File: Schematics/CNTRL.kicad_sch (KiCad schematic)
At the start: 14 parts, among them SW1 RotaryEncoder_Switch, SW2 RotaryEncoder_Switch, SW3 RotaryEncoder_Switch, U5 MCP23017_SP

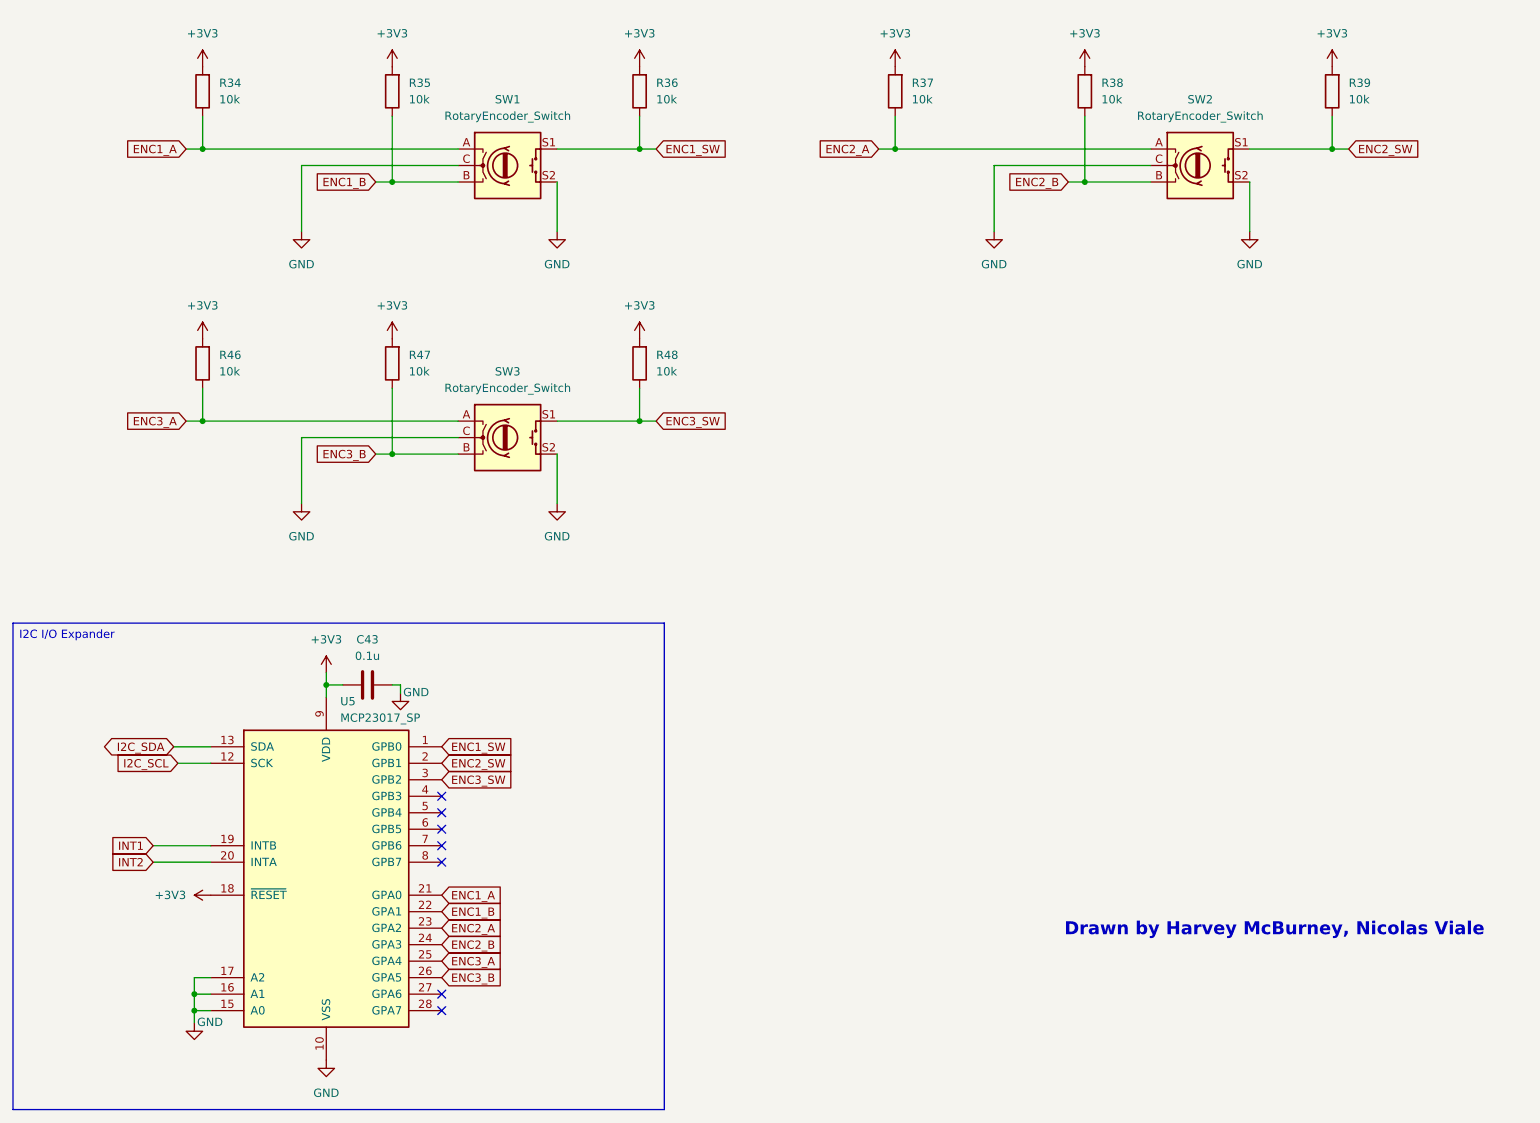
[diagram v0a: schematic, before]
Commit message: Tidied up Schematic
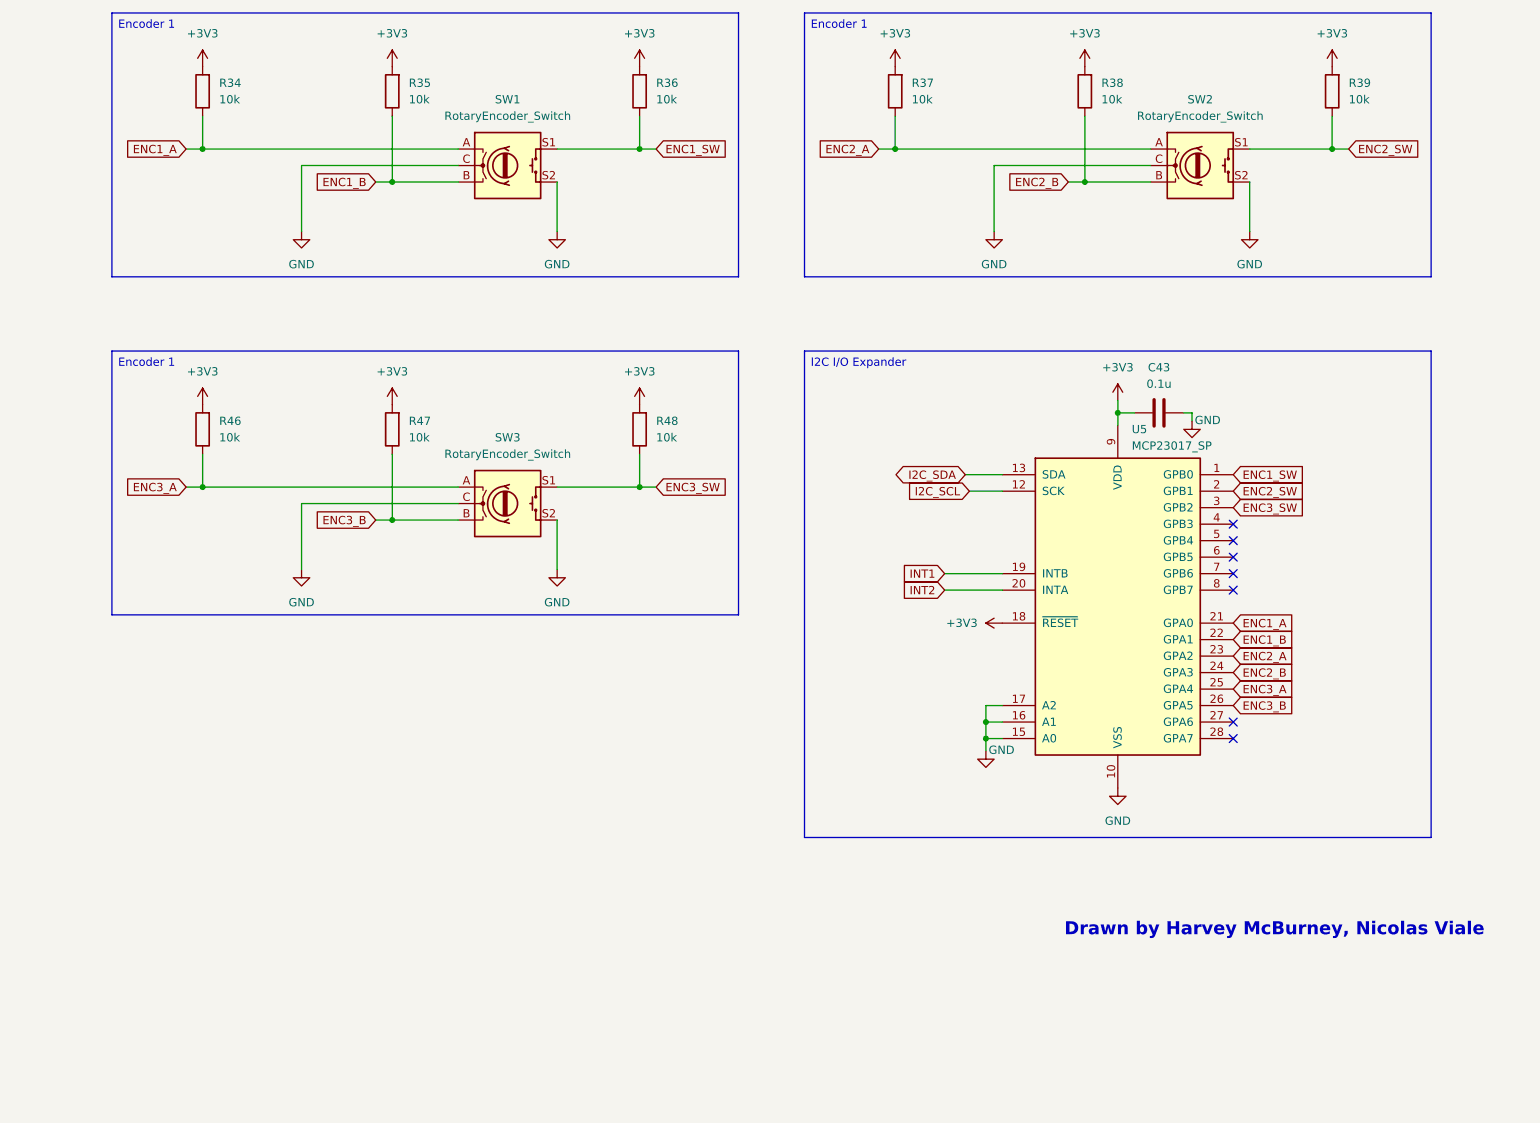
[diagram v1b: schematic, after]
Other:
- moved on the sheet: C43, R46, R47, R48, SW3, U5
